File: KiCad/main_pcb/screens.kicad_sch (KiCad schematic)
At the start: 21 parts, among them U11 TI TXB0104DR, U12 ILI9488, U13 TI TXB0104DR, U14 SD Card Socket, U16 TI TXB0104DR

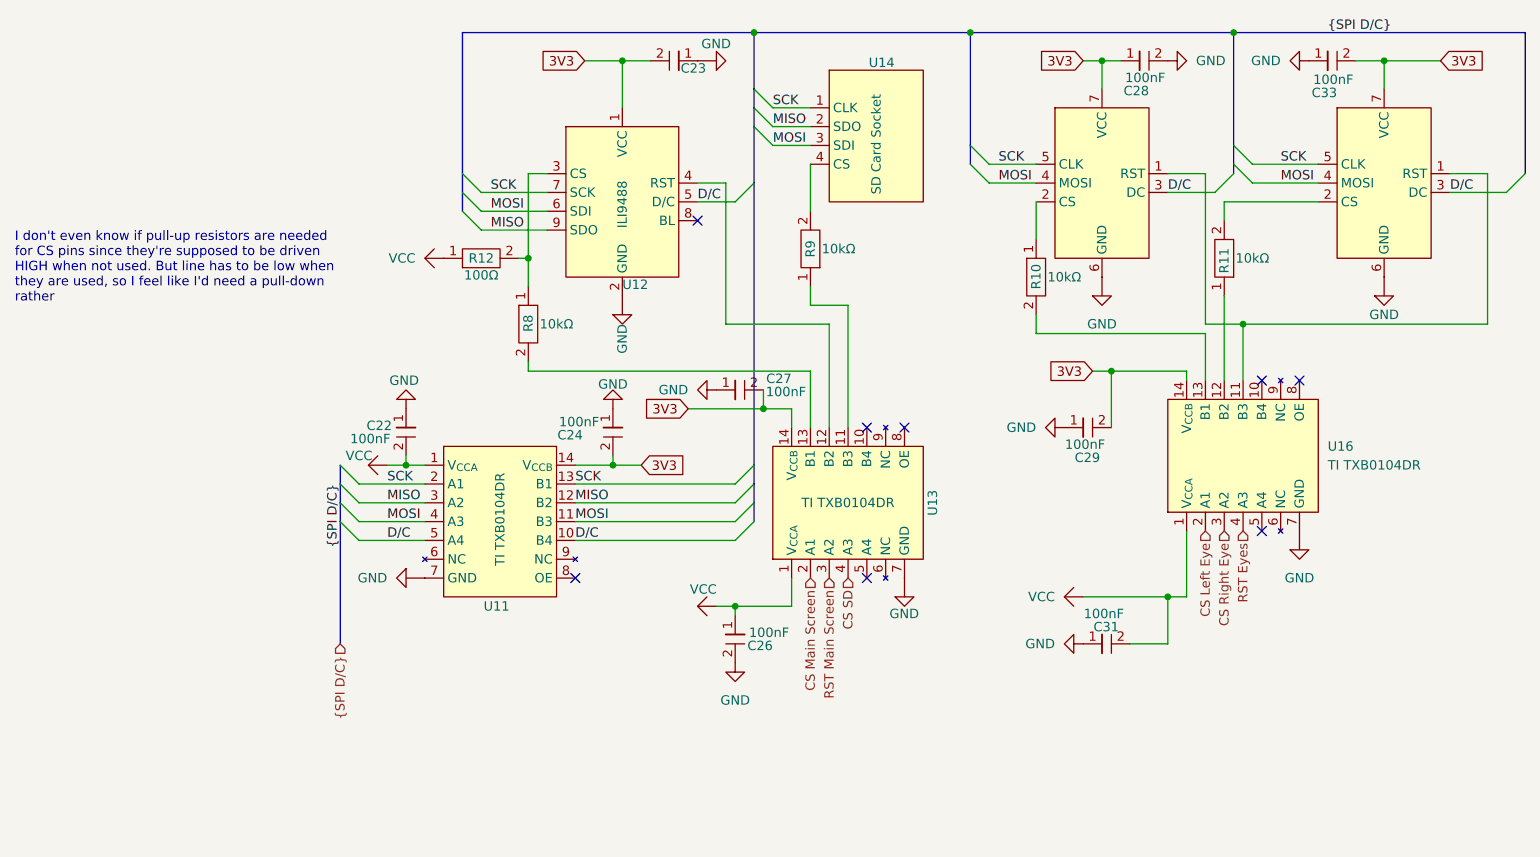
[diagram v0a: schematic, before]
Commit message: feat(KiCad): Continues work
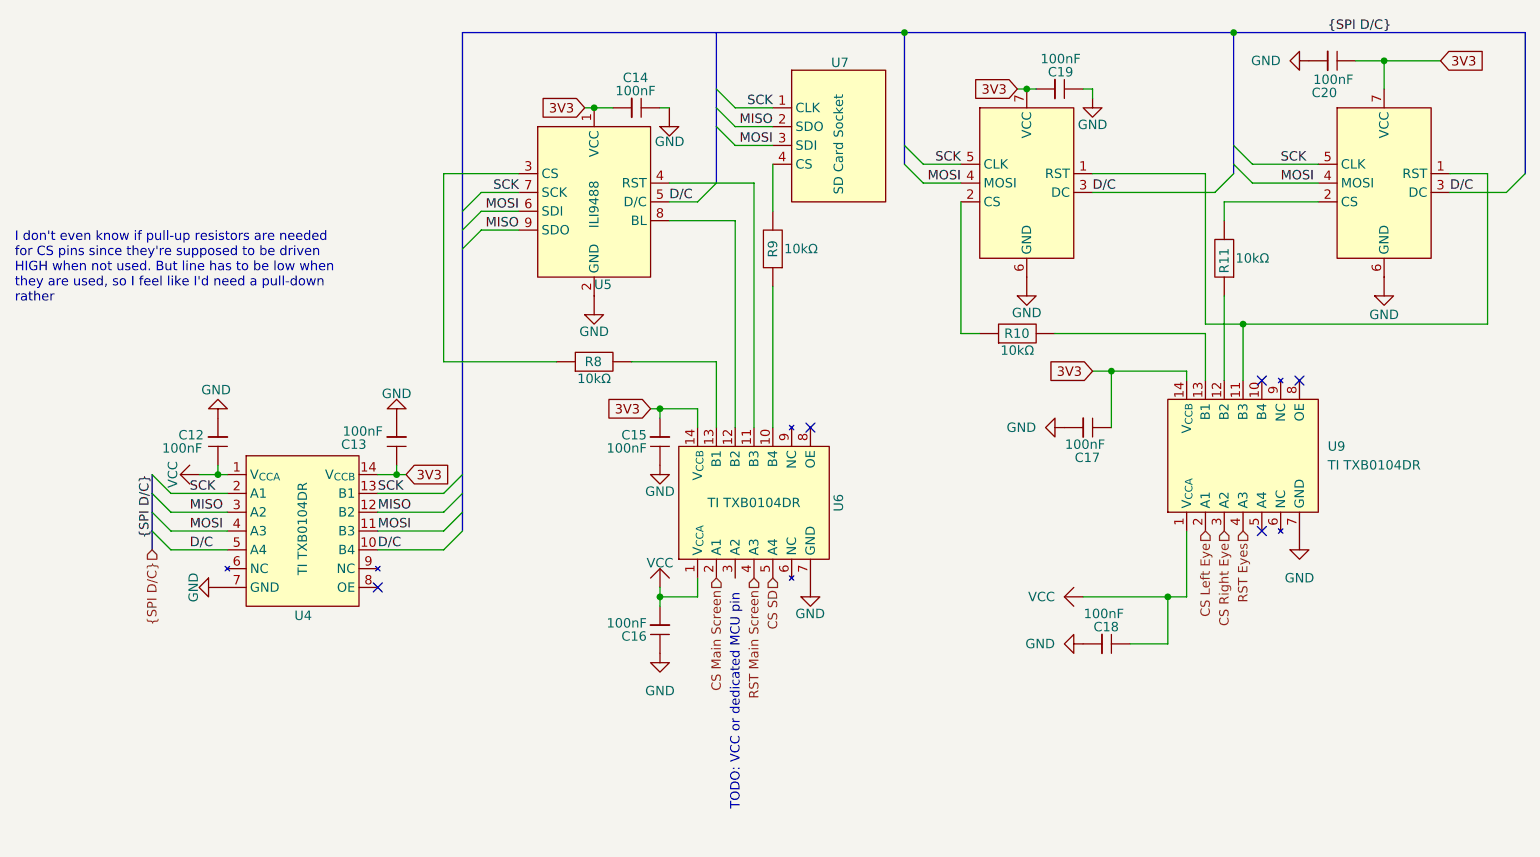
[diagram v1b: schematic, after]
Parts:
- removed C23: 100nF, Capacitor_SMD:C_0201_0603Metric_Pad0.64x0.40mm_HandSolder, symbol Lily's Pad:Capacitor
- removed R12: 100Ω, Resistor_SMD:R_0201_0603Metric_Pad0.64x0.40mm_HandSolder, symbol Lily's Pad:Resistor
- added C14: 100nF, Capacitor_SMD:C_0201_0603Metric_Pad0.64x0.40mm_HandSolder, symbol Lily's Pad:Capacitor
- renumbered C22 to C12, C24 to C13, C27 to C15, C26 to C16, C29 to C17, C31 to C18, C28 to C19, C33 to C20, U17 to U10, U11 to U4, U12 to U5, U13 to U6, U14 to U7, U15 to U8, U16 to U9
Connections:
- net 3V3: now also C15.1, C14.1; no longer C15.2
- net CS SD: now also U6.5 (A4); no longer U6.4 (A3)
- net GND: now also C15.2, C14.2; no longer C15.1
- net RST Main Screen: now also U6.4 (A3); no longer U6.3 (A2)
- net at R9.1: now also U6.10 (B4); no longer U6.11 (B3)
- net at U5.4 (RST): now also U6.11 (B3); no longer U6.12 (B2)
- net at U5.8 (BL): now also U6.12 (B2)
- no-connect marks 8 -> 5
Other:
- note added: "TODO: VCC or dedicated MCU pin"
- moved on the sheet: U4, U5, U6, U7
